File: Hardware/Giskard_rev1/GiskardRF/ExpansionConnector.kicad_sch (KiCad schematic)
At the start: 8 parts, among them J107 Conn_02x05_Odd_Even, U108 AP22802AW5-7

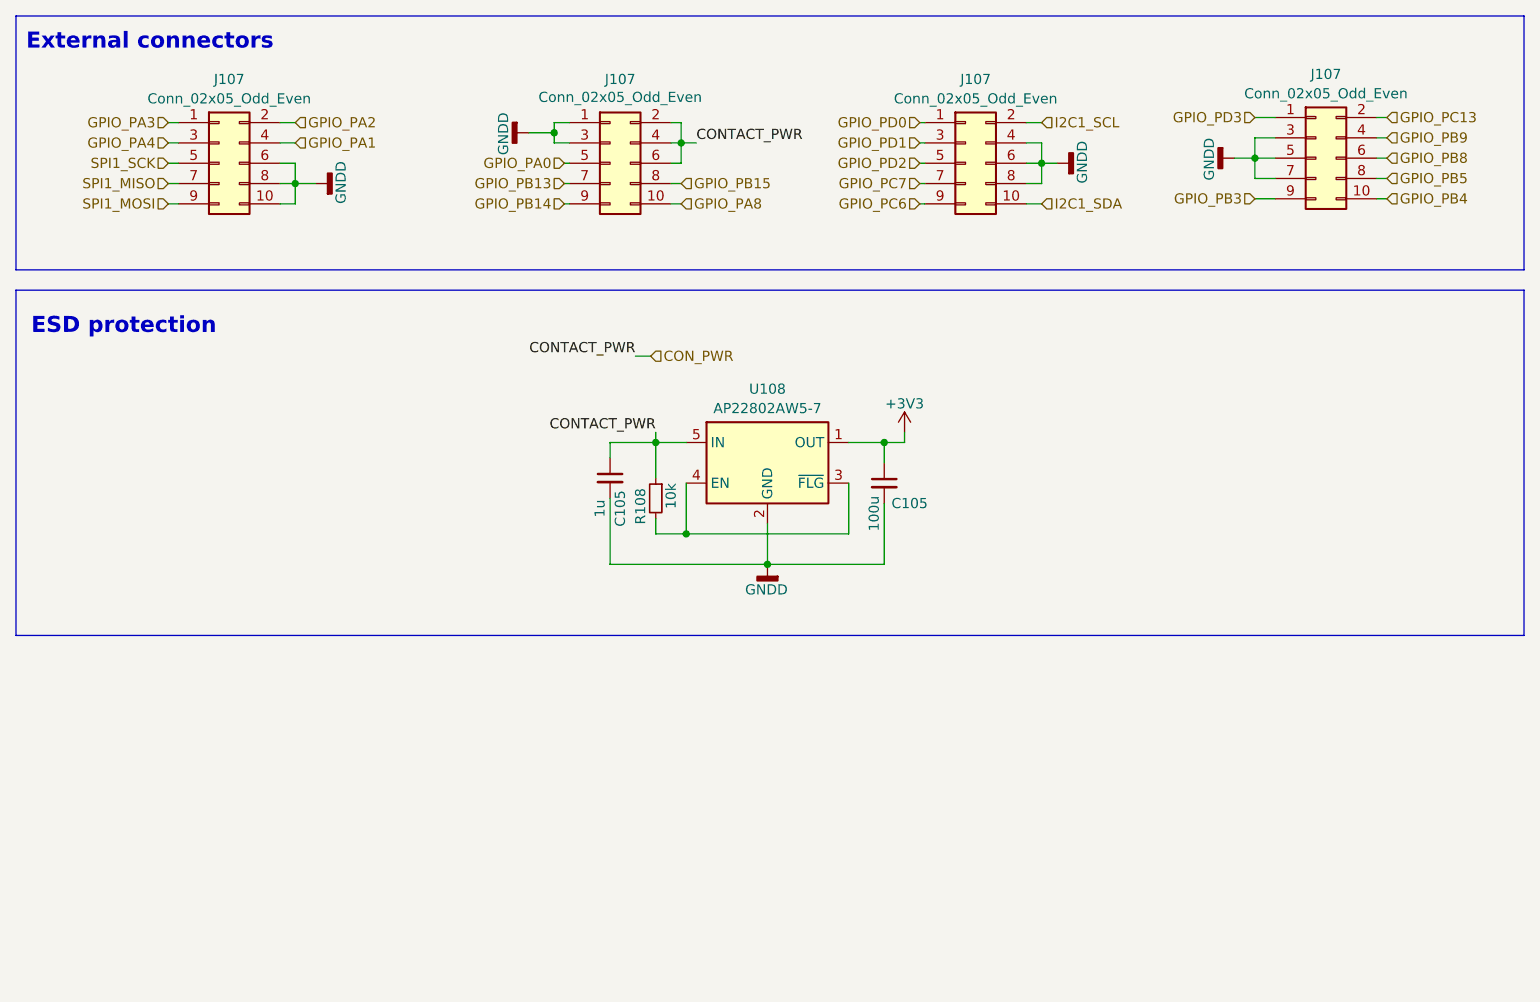
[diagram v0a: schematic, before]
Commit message: Layout dev part 3
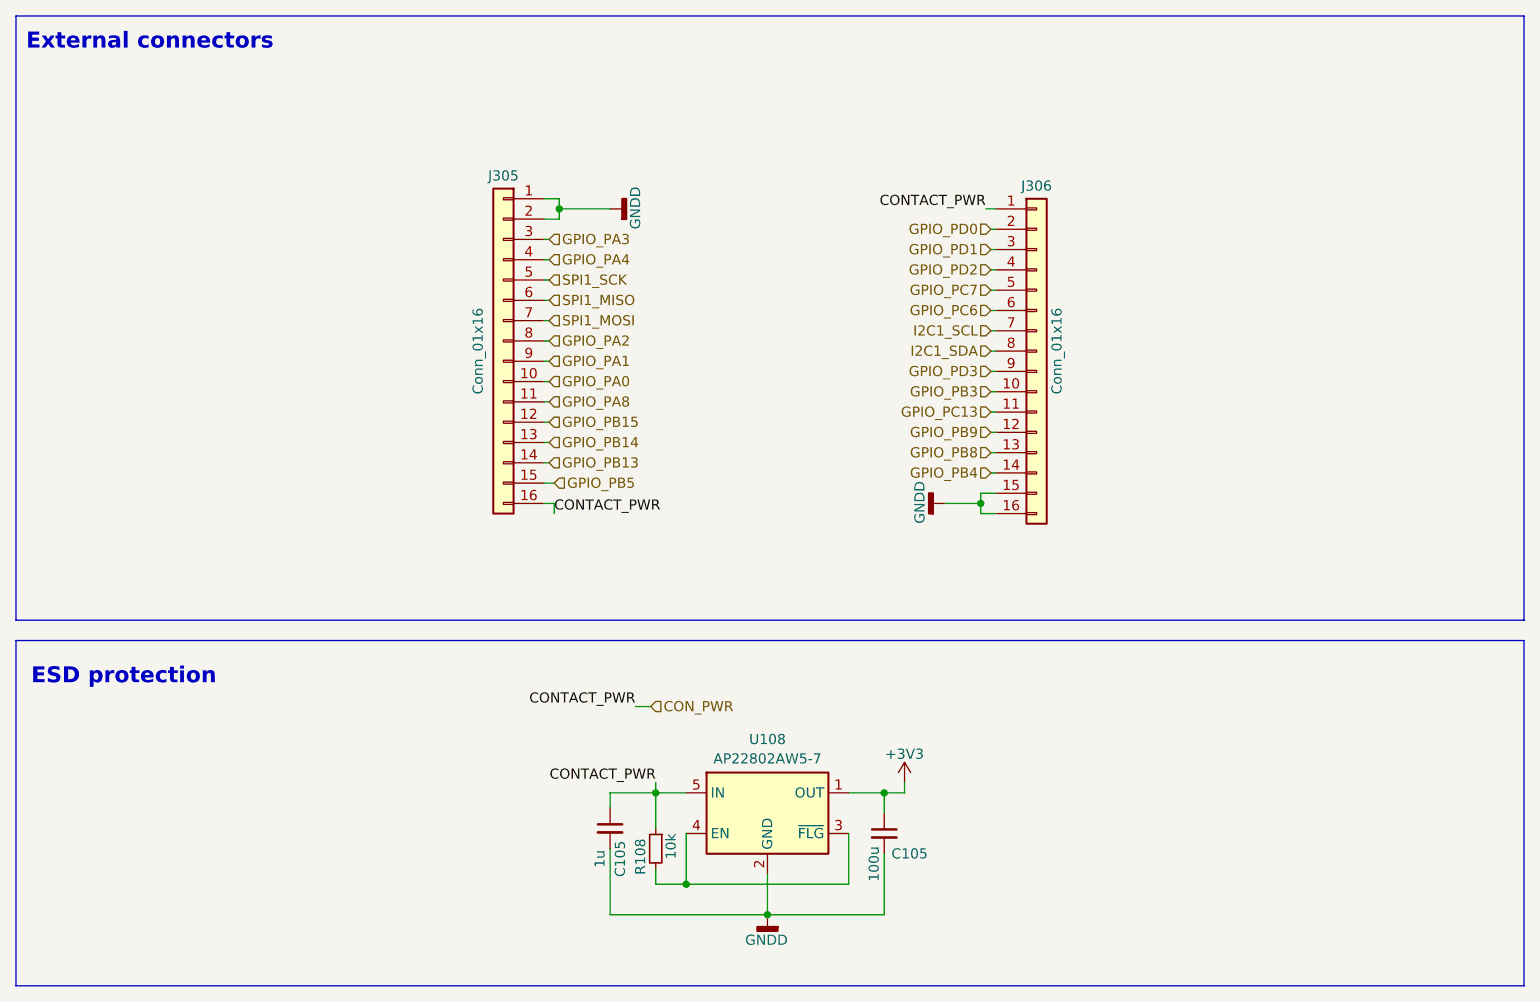
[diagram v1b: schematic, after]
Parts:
- removed J107 (x4): Conn_02x05_Odd_Even, Connector_PinHeader_1.27mm:PinHeader_2x05_P1.27mm_Vertical_SMD, symbol Connector_Generic:Conn_02x05_Odd_Even
- added J305, J306: Conn_01x16, Connector_PinHeader_2.54mm:PinHeader_1x16_P2.54mm_Vertical_SMD_Pin1Left, symbol Connector_Generic:Conn_01x16
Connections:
- net CON_PWR: now also J305.16 (Pin_16), J306.1 (Pin_1)
- net GNDD: now also J305.1 (Pin_1), J305.2 (Pin_2), J306.15 (Pin_15), J306.16 (Pin_16)
- net GPIO_PA0: now also J305.10 (Pin_10)
- net GPIO_PA1: now also J305.9 (Pin_9)
- net GPIO_PA2: now also J305.8 (Pin_8)
- net GPIO_PA3: now also J305.3 (Pin_3)
- net GPIO_PA4: now also J305.4 (Pin_4)
- net GPIO_PA8: now also J305.11 (Pin_11)
- net GPIO_PB13: now also J305.14 (Pin_14)
- net GPIO_PB14: now also J305.13 (Pin_13)
- net GPIO_PB15: now also J305.12 (Pin_12)
- net GPIO_PB3: now also J306.10 (Pin_10)
- net GPIO_PB4: now also J306.14 (Pin_14)
- net GPIO_PB5: now also J305.15 (Pin_15)
- net GPIO_PB8: now also J306.13 (Pin_13)
- net GPIO_PB9: now also J306.12 (Pin_12)
- net GPIO_PC13: now also J306.11 (Pin_11)
- net GPIO_PC6: now also J306.6 (Pin_6)
- net GPIO_PC7: now also J306.5 (Pin_5)
- net GPIO_PD0: now also J306.2 (Pin_2)
- net GPIO_PD1: now also J306.3 (Pin_3)
- net GPIO_PD2: now also J306.4 (Pin_4)
- net GPIO_PD3: now also J306.9 (Pin_9)
- net I2C1_SCL: now also J306.7 (Pin_7)
- net I2C1_SDA: now also J306.8 (Pin_8)
- net SPI1_MISO: now also J305.6 (Pin_6)
- net SPI1_MOSI: now also J305.7 (Pin_7)
- net SPI1_SCK: now also J305.5 (Pin_5)
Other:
- moved on the sheet: C105, R108, U108
